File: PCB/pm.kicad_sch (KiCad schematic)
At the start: 2 parts, among them J2 USB_C_Receptacle_USB2.0_14P, U2 TP4057

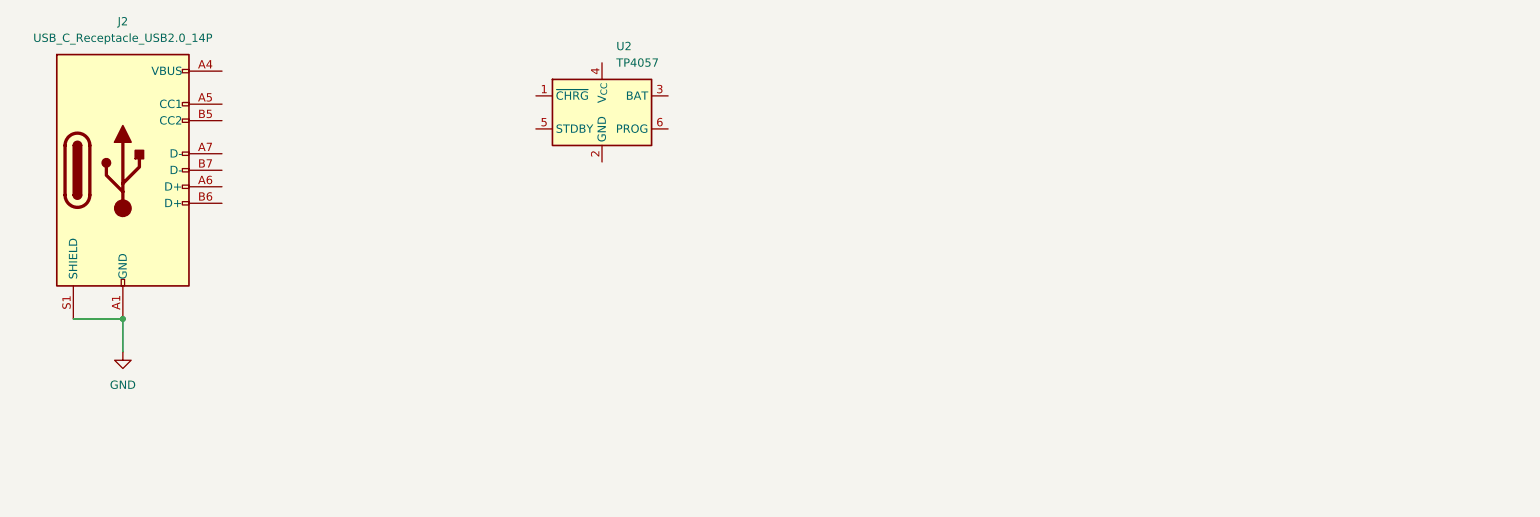
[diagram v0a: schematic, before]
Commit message: Made first PCB
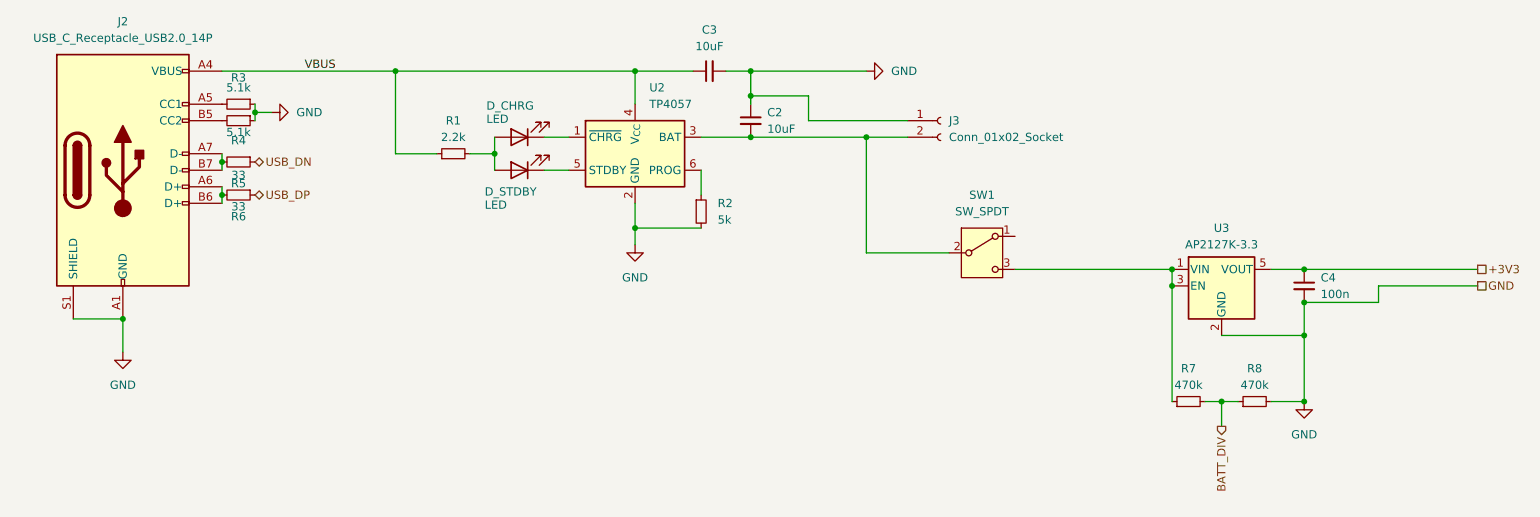
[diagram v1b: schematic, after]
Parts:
- added C2, C3: 10uF, Capacitor_SMD:C_0402_1005Metric, symbol Device:C_Small
- added C4: 100n, Capacitor_SMD:C_0402_1005Metric, symbol Device:C_Small
- added D_CHRG, D_STDBY: LED, LED_SMD:LED_0603_1608Metric, symbol Device:LED
- added J3: Conn_01x02_Socket, Connector_PinHeader_2.54mm:PinHeader_1x02_P2.54mm_Horizontal, symbol Connector:Conn_01x02_Socket
- added R1: 2.2k, Resistor_SMD:R_0402_1005Metric, symbol Device:R_Small
- added R2: 5k, Resistor_SMD:R_0402_1005Metric, symbol Device:R_Small
- added R3, R4: 5.1k, Resistor_SMD:R_0402_1005Metric, symbol Device:R_Small
- added R5, R6: 33, Resistor_SMD:R_0402_1005Metric, symbol Device:R_Small
- added R7, R8: 470k, Resistor_SMD:R_0402_1005Metric, symbol Device:R_Small
- added SW1: SW_SPDT, Button_Switch_SMD:SW_SPDT_PCM12, symbol Switch:SW_SPDT
- added U3: AP2127K-3.3, Package_TO_SOT_SMD:SOT-23-5, symbol Regulator_Linear:AP2127K-3.3
- J2: footprint (none) -> Connector_USB:USB_C_Receptacle_G-Switch_GT-USB-7010ASV
- U2: footprint Package_TO_SOT_SMD:TSOT-23-5 -> Package_TO_SOT_SMD:TSOT-23-6
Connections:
- net GND: now also U2.2 (GND), C2.1, C3.2, C4.2, J3.1 (Pin_1), R2.2, R3.1, R4.1, R8.2, U3.2 (GND)
- net VBUS: now reaches J2.A4 (VBUS), J2.A9 (VBUS), J2.B4 (VBUS), J2.B9 (VBUS)
- net VBUS: now also U2.4 (V_{CC}), C3.1, R1.1
- net at J2.A5 (CC1): now also R3.2
- net at J2.A6 (D+): now also J2.B6 (D+), R6.2
- net at J2.A7 (D-): now also J2.B7 (D-), R5.2
- net at J2.B5 (CC2): now also R4.2
- net at U2.1 (~{CHRG}): now also D_CHRG.1 (K)
- net at U2.3 (BAT): now also C2.2, J3.2 (Pin_2), SW1.2 (B)
- net at U2.5 (STDBY): now also D_STDBY.1 (K)
- net at U2.6 (PROG): now also R2.1
- new net: D_CHRG.2 (A), D_STDBY.2 (A), R1.2
- new net: R7.1, SW1.3 (C), U3.1 (VIN), U3.3 (EN)
- new net +3V3: C4.1, U3.5 (VOUT)
- new net BATT_DIV: R7.2, R8.1
- new net USB_DN: R5.1
- new net USB_DP: R6.1
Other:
- moved on the sheet: U2
